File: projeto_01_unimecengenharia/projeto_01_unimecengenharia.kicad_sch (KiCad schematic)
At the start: 2 parts

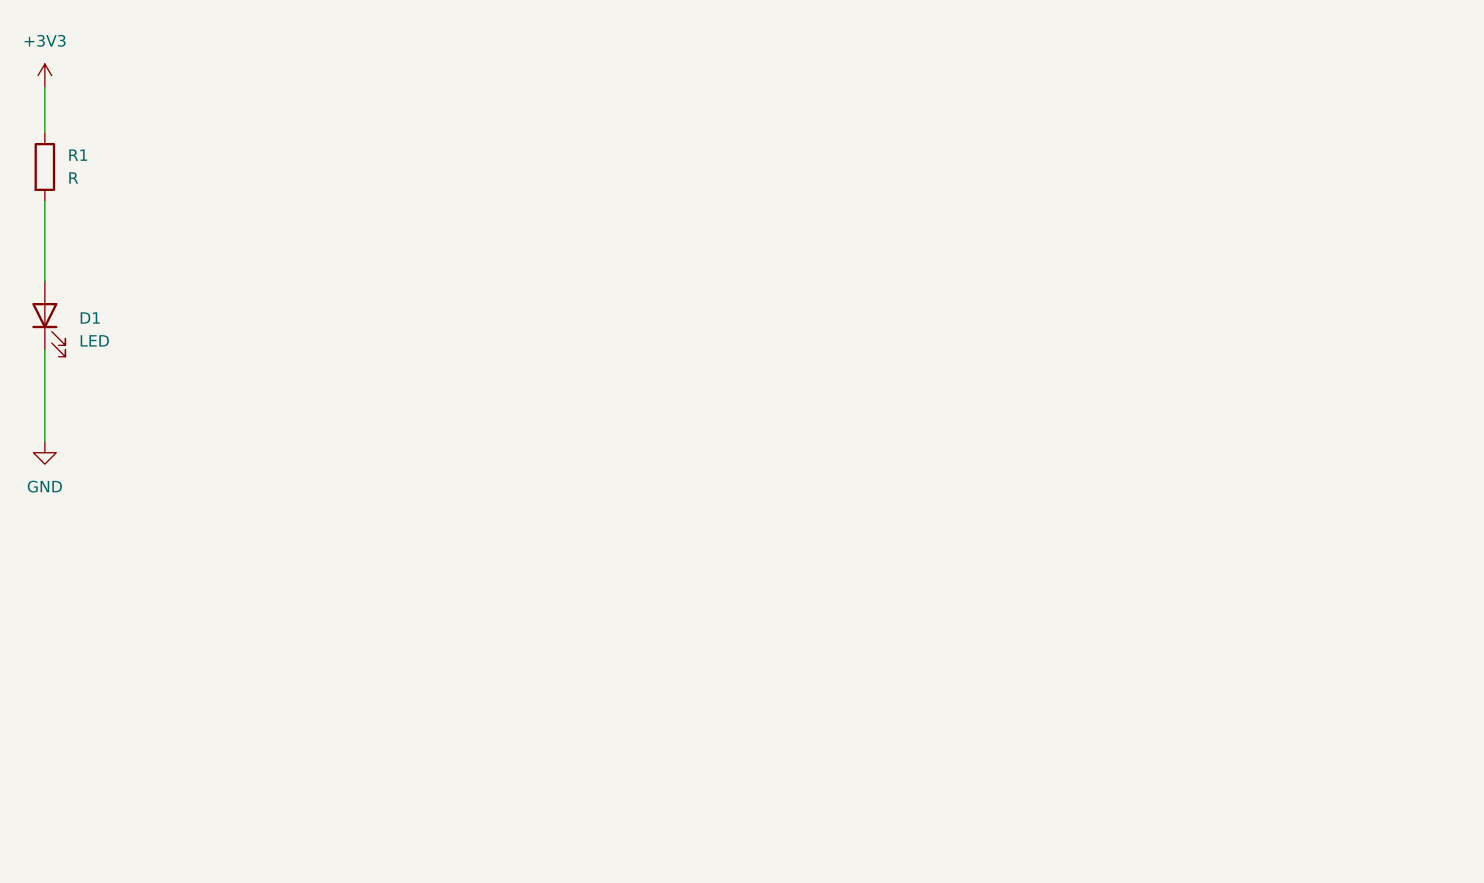
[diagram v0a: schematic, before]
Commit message: mais alguns ajustes
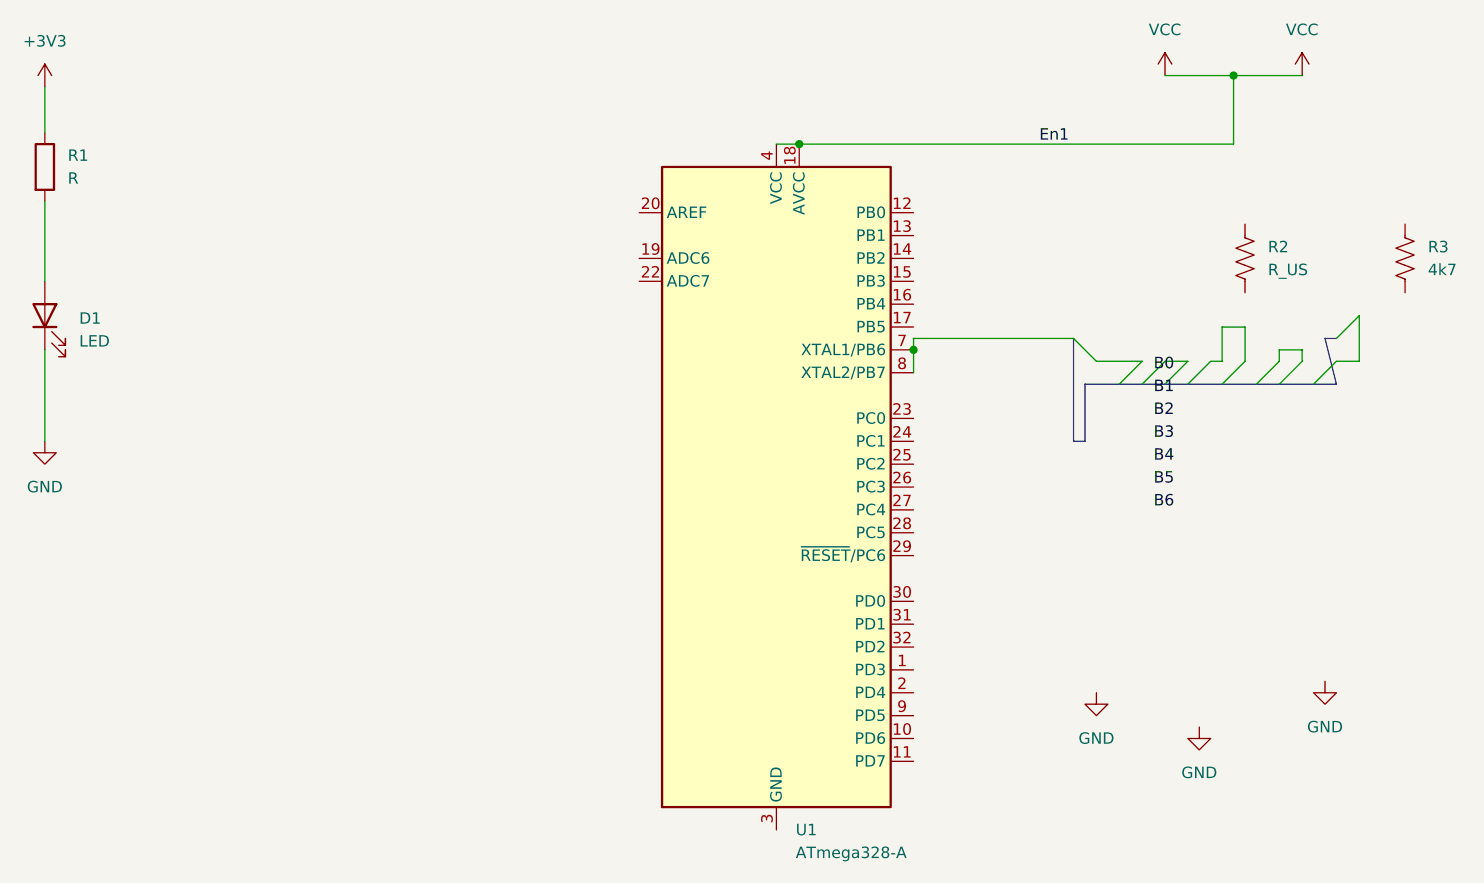
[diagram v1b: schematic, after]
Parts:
- added R2: R_US, symbol Device:R_US
- added R3: 4k7, symbol Device:R_US
- added U1: ATmega328-A, Package_QFP:TQFP-32_7x7mm_P0.8mm, symbol MCU_Microchip_ATmega:ATmega328-A
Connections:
- new net: U1.21 (GND), U1.3 (GND), U1.5 (GND)
- new net: U1.7 (XTAL1/PB6), U1.8 (XTAL2/PB7)
- new net VCC: U1.18 (AVCC), U1.4 (VCC), U1.6 (VCC)

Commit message: Apaguei tudo
Vamos começar a projetar de verdade
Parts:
- removed D1: LED, symbol Device:LED
- removed R1: R, symbol Device:R
- removed R2: R_US, symbol Device:R_US
- removed R3: 4k7, symbol Device:R_US
- removed U1: ATmega328-A, Package_QFP:TQFP-32_7x7mm_P0.8mm, symbol MCU_Microchip_ATmega:ATmega328-A
